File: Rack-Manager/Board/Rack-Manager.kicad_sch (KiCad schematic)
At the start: 0 parts

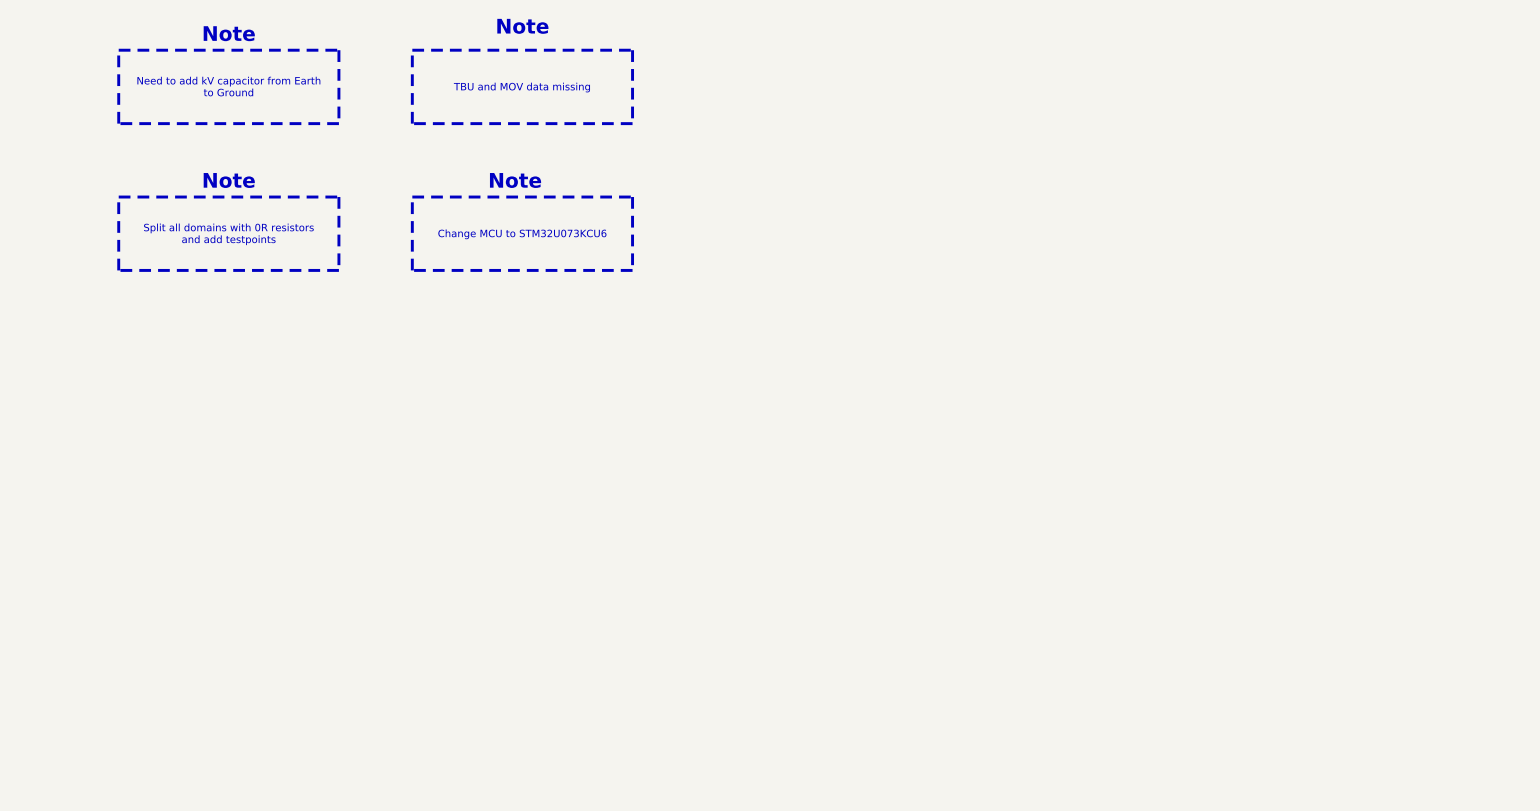
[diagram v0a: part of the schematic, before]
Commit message: Added/Updated notes for TODOs
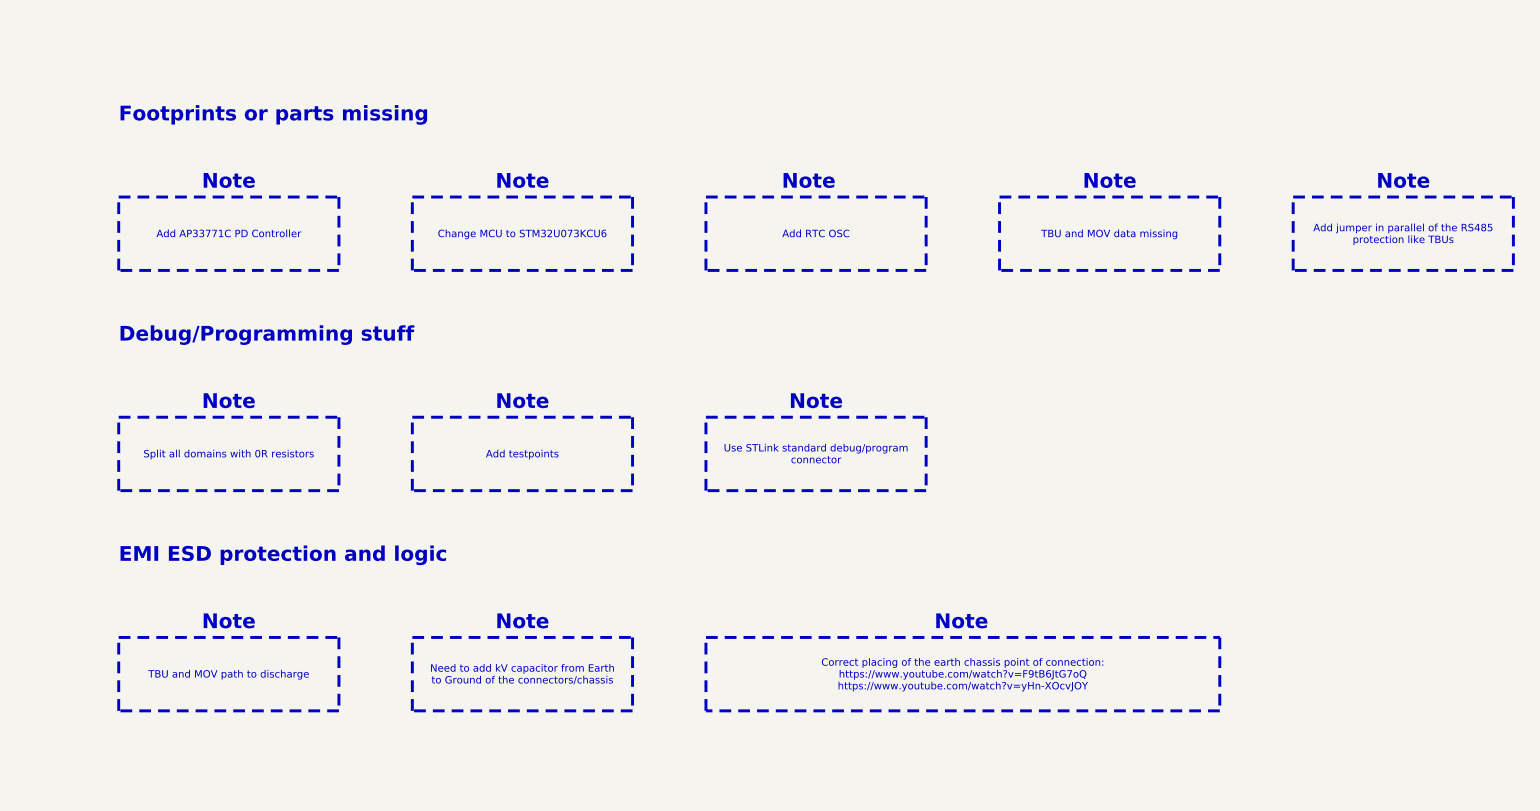
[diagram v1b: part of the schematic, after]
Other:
- note added: "Debug/Programming stuff"
- note added: "EMI ESD protection and logic"
- note added: "Footprints or parts missing"
